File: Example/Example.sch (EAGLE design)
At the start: 5 parts

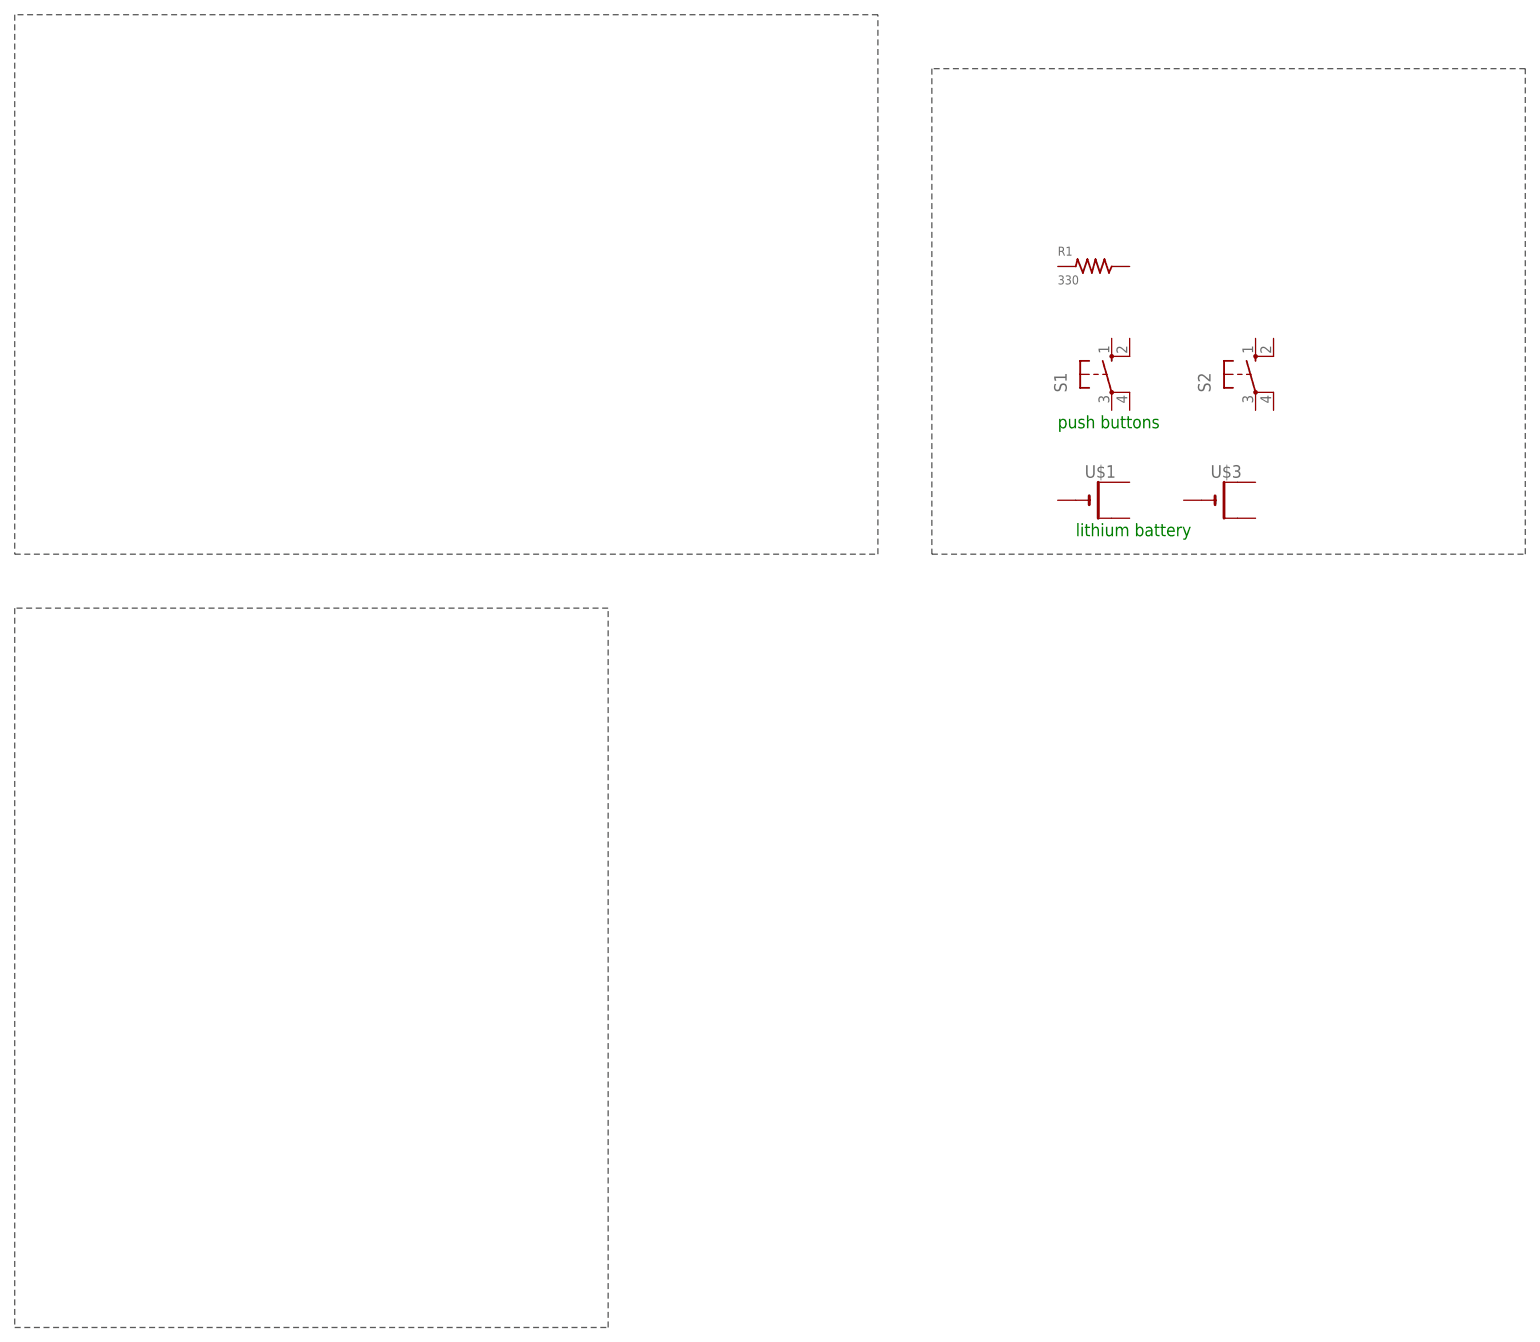
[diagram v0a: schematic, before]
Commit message: Revert "add"
This reverts commit c6e4ebc28e4f55c76fdda87922b953a09ff3b68b.
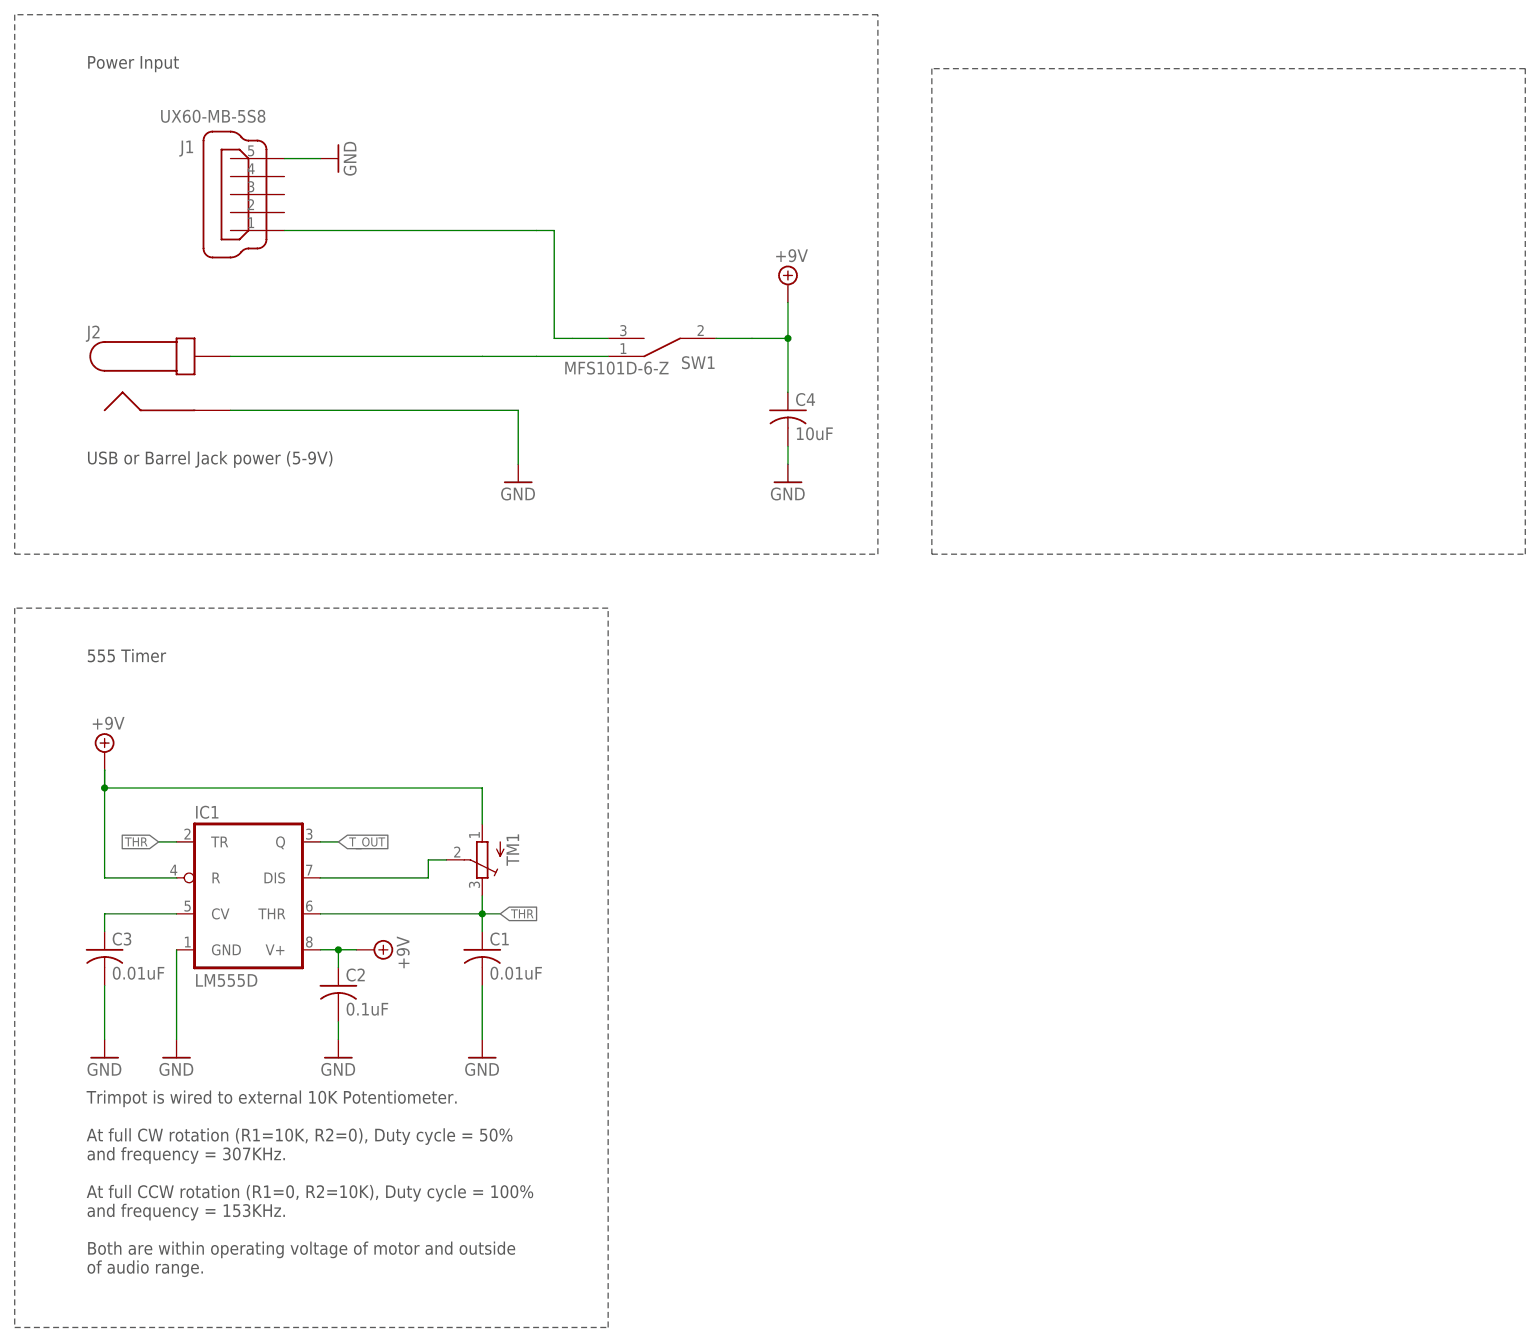
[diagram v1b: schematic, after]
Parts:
- removed R1: 330, RoboJackets-Resistors:GHOST_RESISTOR
- removed S1, S2: (no value), adafruit:40-XX
- removed U$1, U$3: (no value), adafruit:CR1220SMT
- added C1, C3: 0.01uF, rcl:C-USC0603
- added C2: 0.1uF, rcl:C-USC0603
- added C4: 10uF, rcl:C-USC0603
- added IC1: LM555D, adafruit:LM555D
- added J1: UX60-MB-5S8, RoboJackets-Connectors:UX60-MB-5S8
- added J2: (no value), RoboJackets-Connectors:PJ-037A
- added SW1: MFS101D-6-Z, Example:MFS101D-6-Z
- added TM1: (no value), adafruit:TRIMPOT3386
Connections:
- new net +9V: C2.1, C4.1, IC1.R, IC1.V+, SW1.COMMON, TM1.A
- new net GND: C1.2, C2.2, C3.2, C4.2, IC1.GND, J1.5, J2.2
- new net N$1: IC1.DIS, TM1.S
- new net N$3: C3.1, IC1.CV
- new net N$4: J1.1, SW1.B
- new net N$6: J2.1, SW1.A
- new net THR: C1.1, IC1.THR, IC1.TR, TM1.E
- new net T_OUT: IC1.Q
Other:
- note added: "555 Timer"
- note added: "Power Input"
- note added: "Trimpot is wired to external 10K Potentiometer. At full CW rotation (R1=10K, R2=0), Duty cycle = 50% and frequency = 307KHz. At full CCW rotation (R1=0, R2=10K), Duty cycle = 100% and frequency = 153KHz. Both are within operating voltage of motor and outside of audio range."
- note added: "USB or Barrel Jack power (5-9V)"
- note removed: "lithium battery"
- note removed: "push buttons"
